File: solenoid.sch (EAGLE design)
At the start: 43 parts, among them U1 QS5K2TR, U2 QS5K2TR, U3 QS5K2TR, U4 QS5K2TR, U5 QS5K2TR, U6 QS5K2TR, Y1 ECS-80-S-4X

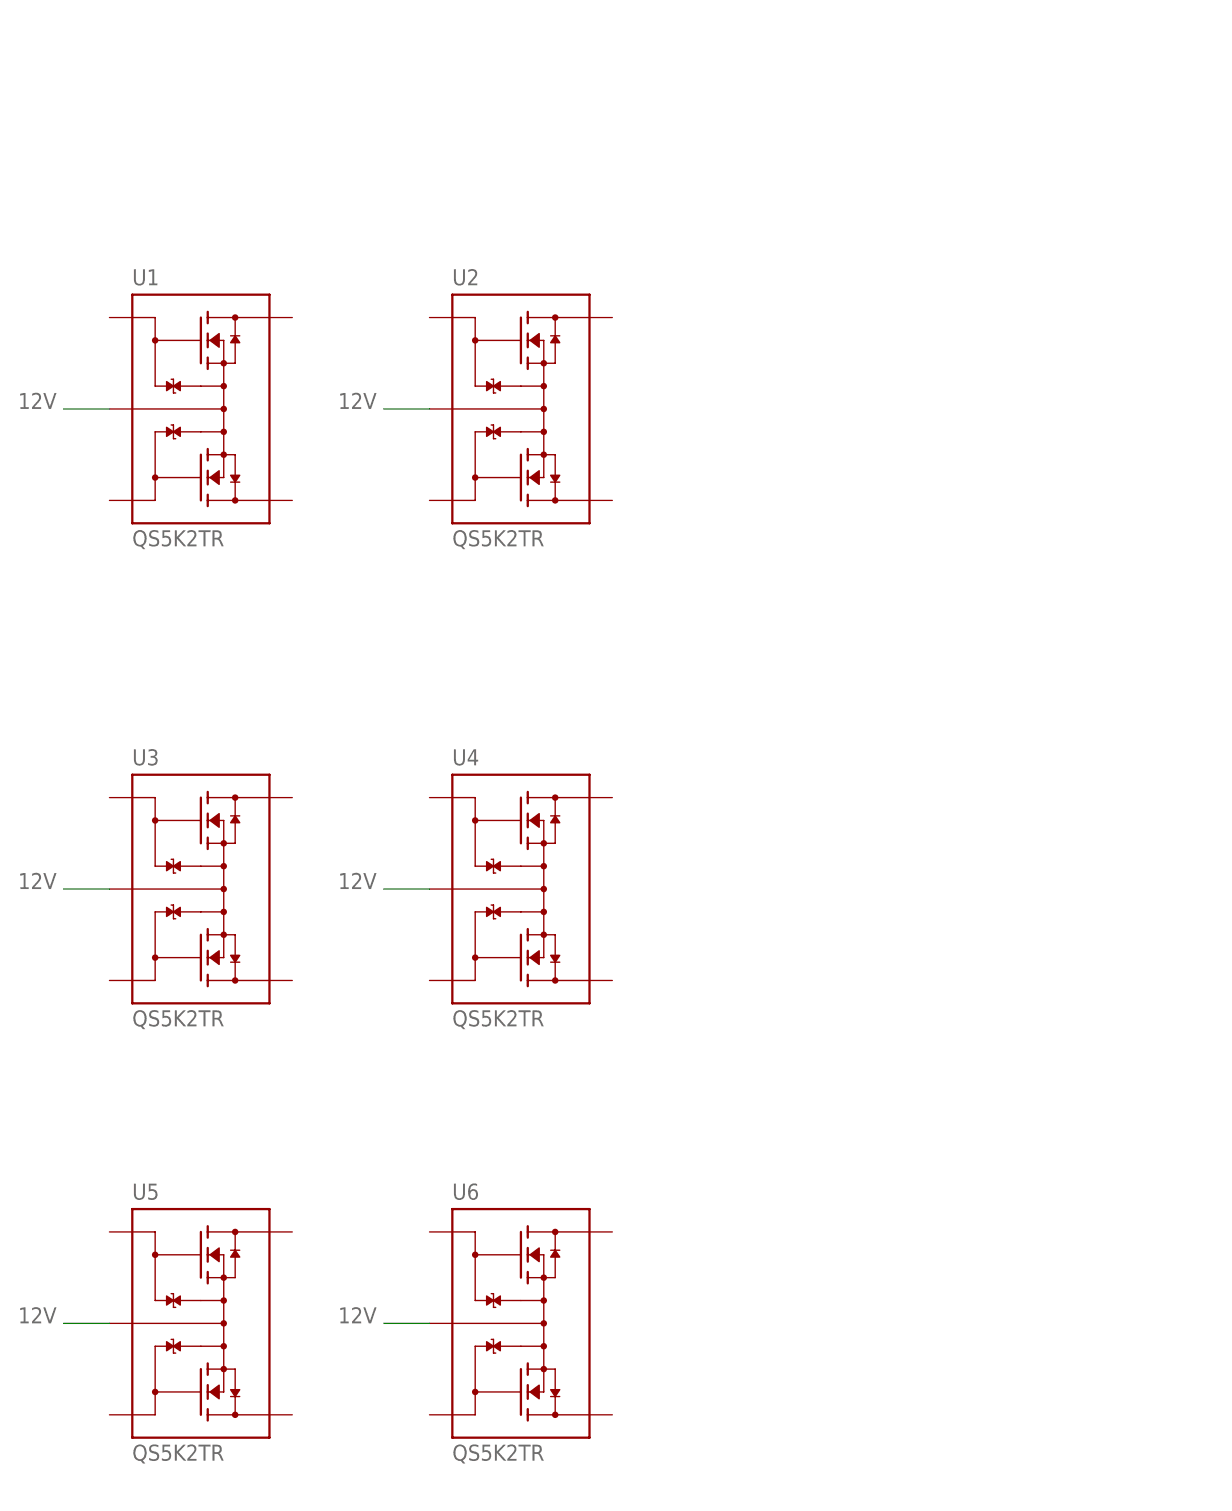
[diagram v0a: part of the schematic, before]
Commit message: potentially finished schematic
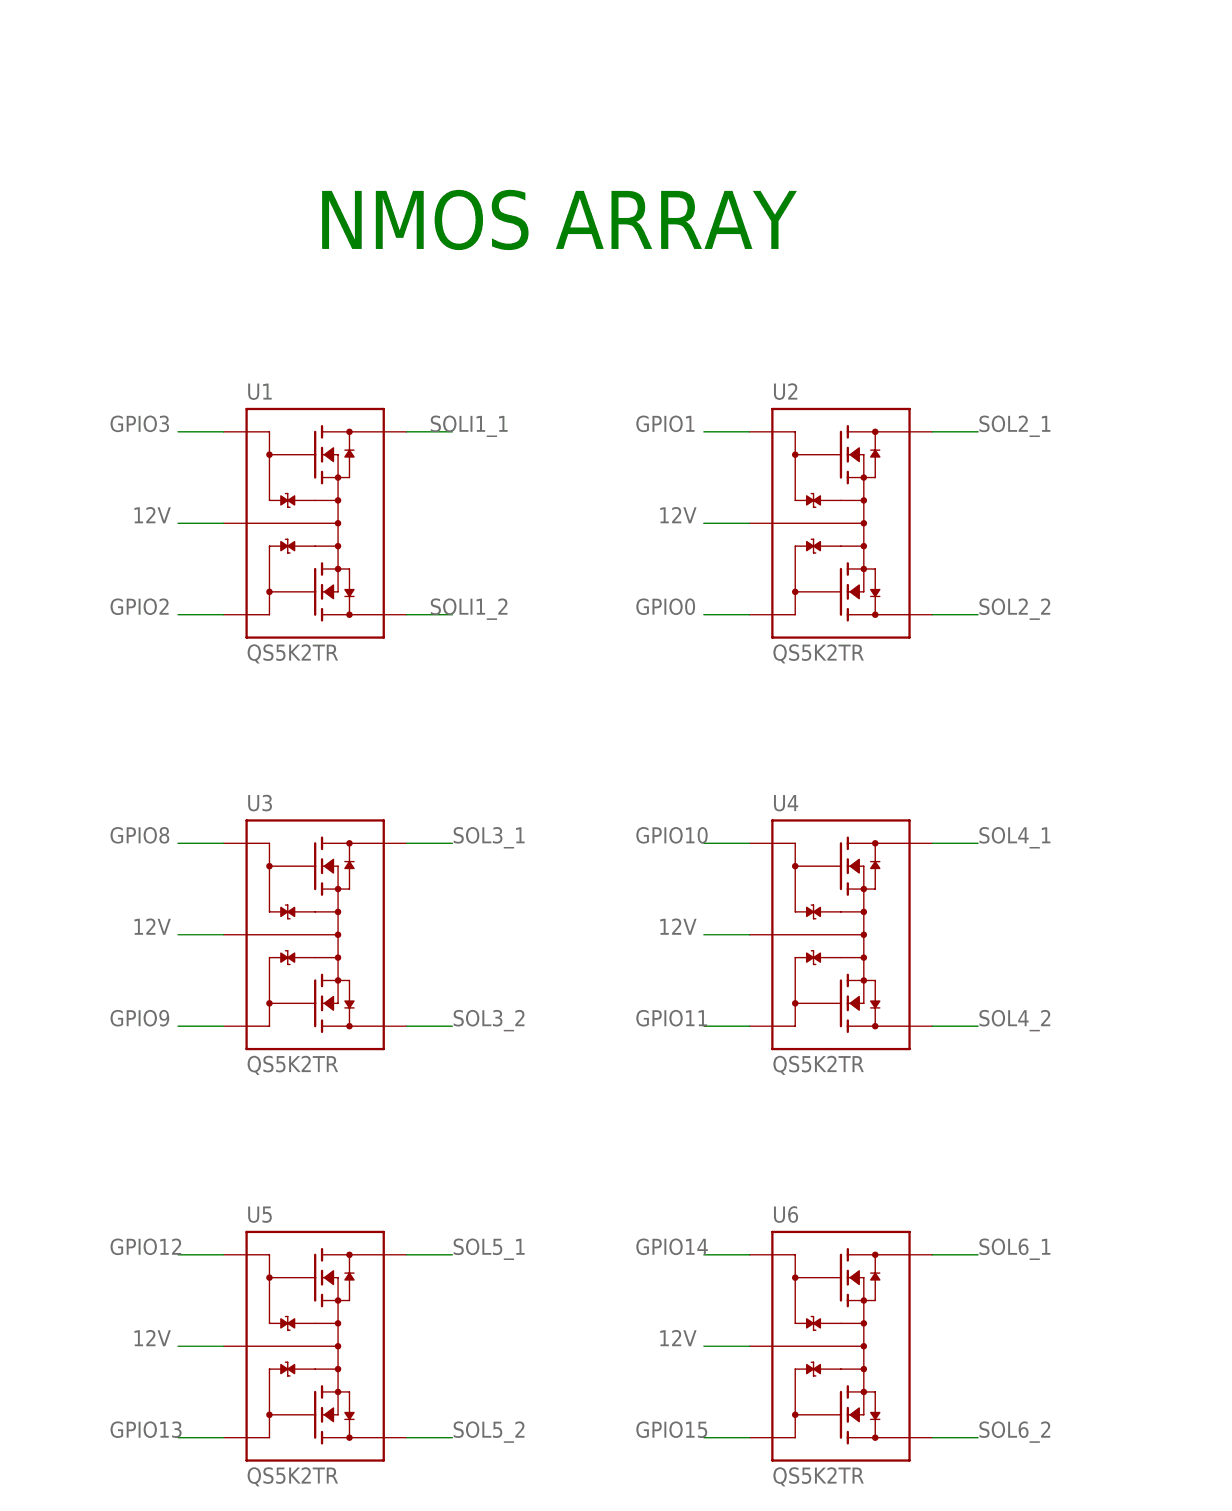
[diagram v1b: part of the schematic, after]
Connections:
- new net SOLI1_1: U1.TR1_DRAIN
- new net SOLI1_2: U1.TR2_DRAIN
- net GPIO0: now also U2.TR2_GATE
- net GPIO1: now also U2.TR1_GATE
- net GPIO10: now also U4.TR1_GATE
- net GPIO11: now also U4.TR2_GATE
- net GPIO12: now also U5.TR1_GATE
- net GPIO13: now also U5.TR2_GATE
- net GPIO14: now also U6.TR1_GATE
- net GPIO15: now also U6.TR2_GATE
- net GPIO2: now also U1.TR2_GATE
- net GPIO3: now also U1.TR1_GATE
- net GPIO8: now also U3.TR1_GATE
- net GPIO9: now also U3.TR2_GATE
- net SOL2_1: now also U2.TR1_DRAIN
- net SOL2_2: now also U2.TR2_DRAIN
- net SOL3_1: now also U3.TR1_DRAIN
- net SOL3_2: now also U3.TR2_DRAIN
- net SOL4_1: now also U4.TR1_DRAIN
- net SOL4_2: now also U4.TR2_DRAIN
- net SOL5_1: now also U5.TR1_DRAIN
- net SOL5_2: now also U5.TR2_DRAIN
- net SOL6_1: now also U6.TR1_DRAIN
- net SOL6_2: now also U6.TR2_DRAIN
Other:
- note added: "NMOS ARRAY"
- moved on the sheet: U1, U2, U3, U4, U5, U6

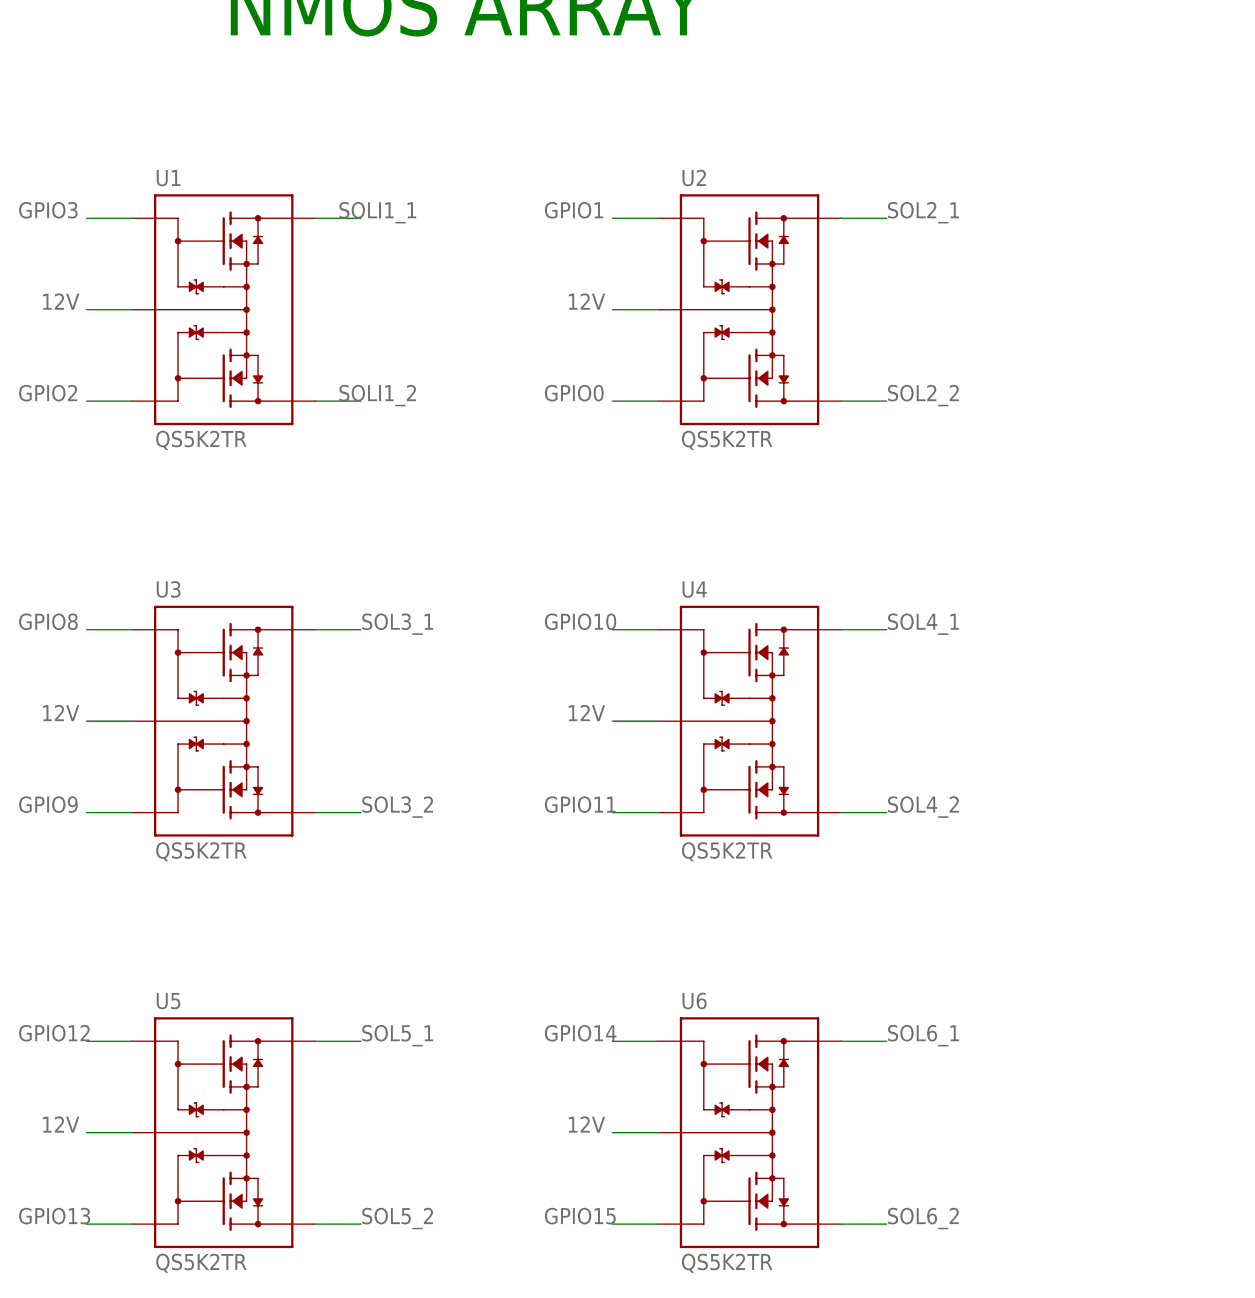
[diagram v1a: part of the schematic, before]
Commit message: solenoid work
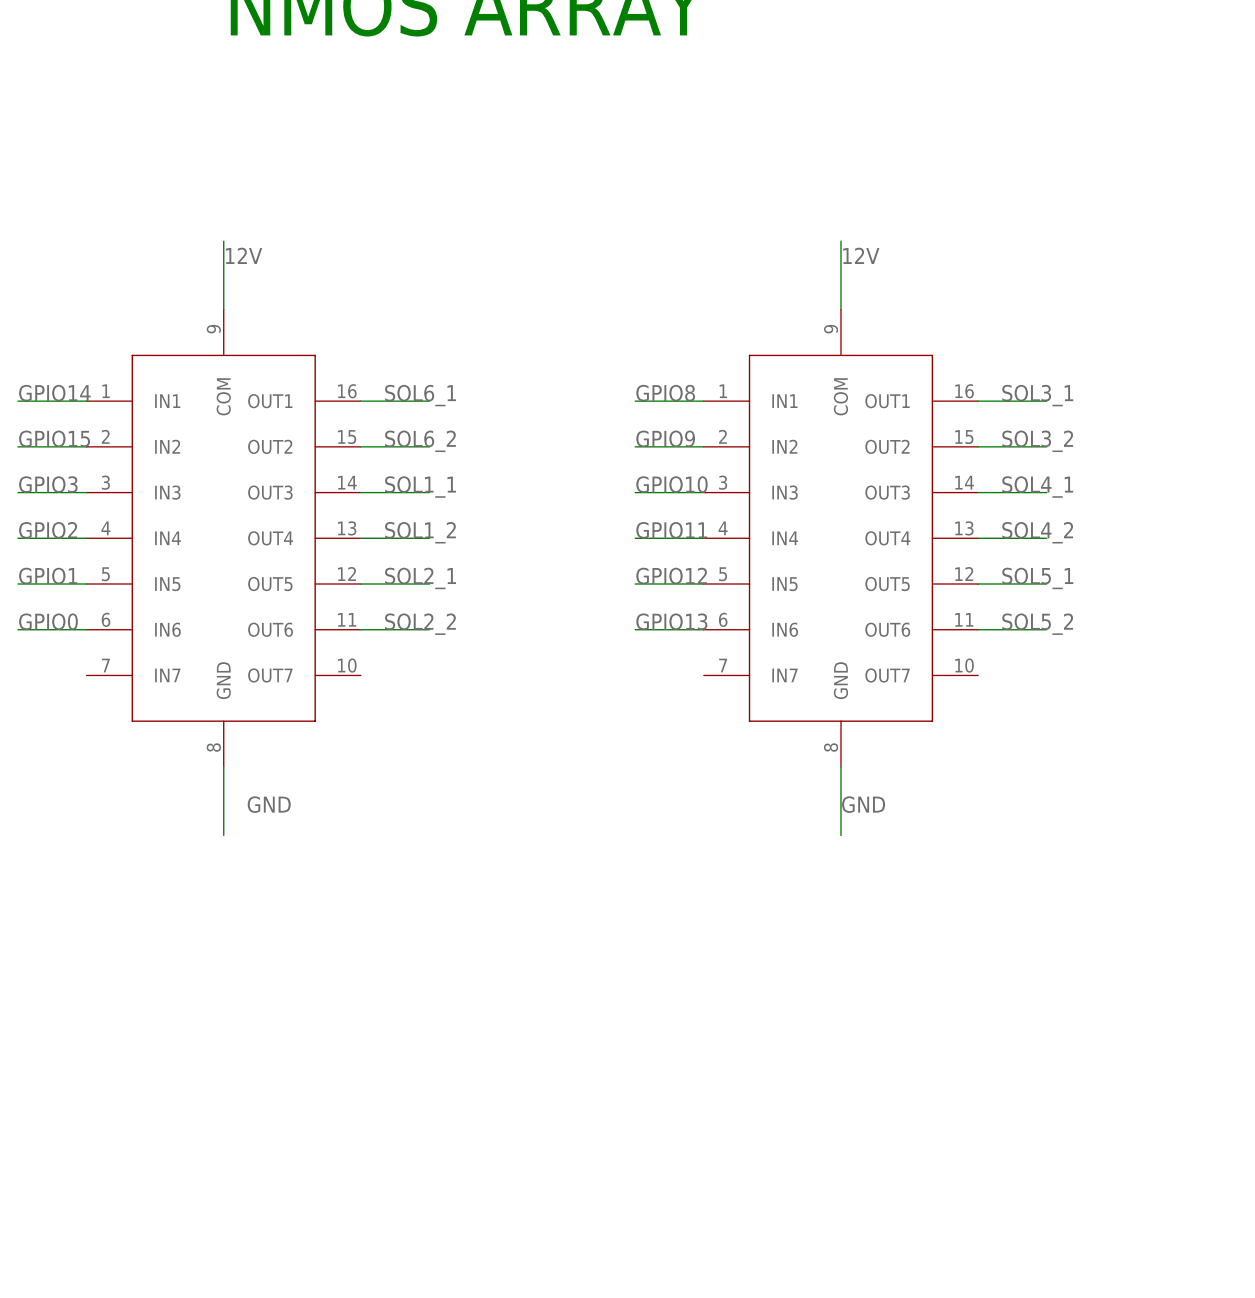
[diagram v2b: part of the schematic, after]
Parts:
- removed U3, U4, U5, U6: QS5K2TR, QS5K2TR:QS5K2TR
- U1, U2: value QS5K2TR -> ULN2003V12; device QS5K2TR:QS5K2TR -> ULN2003V12:ULN2003V12
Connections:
- removed net SOLI1_1: U1.TR1_DRAIN
- removed net SOLI1_2: U1.TR2_DRAIN
- net 12V: now also U1.COM, U2.COM; no longer U1.TR1_TR2_SOURCE, U2.TR1_TR2_SOURCE, U3.TR1_TR2_SOURCE, U4.TR1_TR2_SOURCE, U5.TR1_TR2_SOURCE, U6.TR1_TR2_SOURCE
- net GND: now also U1.GND, U2.GND
- net GPIO0: now also U1.IN6; no longer U2.TR2_GATE
- net GPIO1: now also U1.IN5; no longer U2.TR1_GATE
- net GPIO10: now also U2.IN3; no longer U4.TR1_GATE
- net GPIO11: now also U2.IN4; no longer U4.TR2_GATE
- net GPIO12: now also U2.IN5; no longer U5.TR1_GATE
- net GPIO13: now also U2.IN6; no longer U5.TR2_GATE
- net GPIO14: now also U1.IN1; no longer U6.TR1_GATE
- net GPIO15: now also U1.IN2; no longer U6.TR2_GATE
- net GPIO2: now also U1.IN4; no longer U1.TR2_GATE
- net GPIO3: now also U1.IN3; no longer U1.TR1_GATE
- net GPIO8: now also U2.IN1; no longer U3.TR1_GATE
- net GPIO9: now also U2.IN2; no longer U3.TR2_GATE
- net SOL1_1: now also U1.OUT3
- net SOL1_2: now also U1.OUT4
- net SOL2_1: now also U1.OUT5; no longer U2.TR1_DRAIN
- net SOL2_2: now also U1.OUT6; no longer U2.TR2_DRAIN
- net SOL3_1: now also U2.OUT1; no longer U3.TR1_DRAIN
- net SOL3_2: now also U2.OUT2; no longer U3.TR2_DRAIN
- net SOL4_1: now also U2.OUT3; no longer U4.TR1_DRAIN
- net SOL4_2: now also U2.OUT4; no longer U4.TR2_DRAIN
- net SOL5_1: now also U2.OUT5; no longer U5.TR1_DRAIN
- net SOL5_2: now also U2.OUT6; no longer U5.TR2_DRAIN
- net SOL6_1: now also U1.OUT1; no longer U6.TR1_DRAIN
- net SOL6_2: now also U1.OUT2; no longer U6.TR2_DRAIN

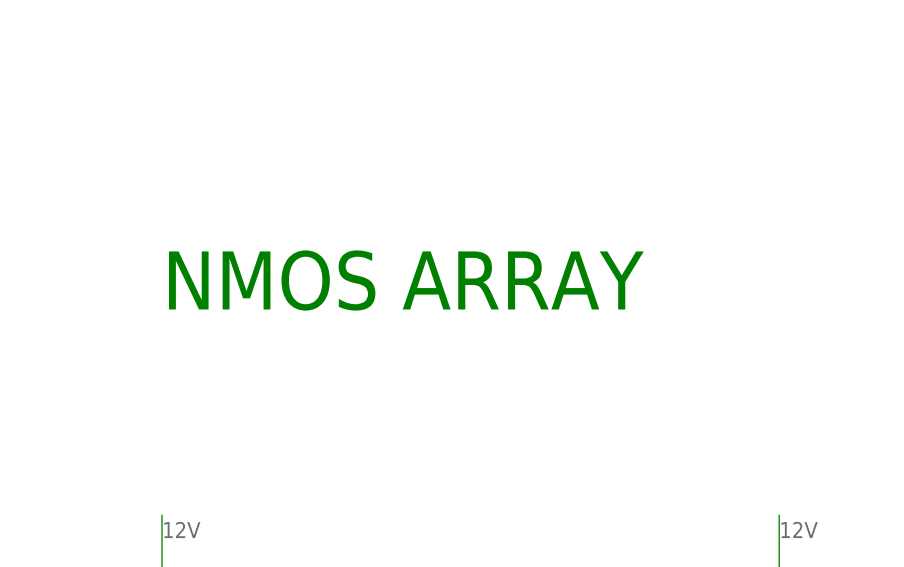
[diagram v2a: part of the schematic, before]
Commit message: uwu
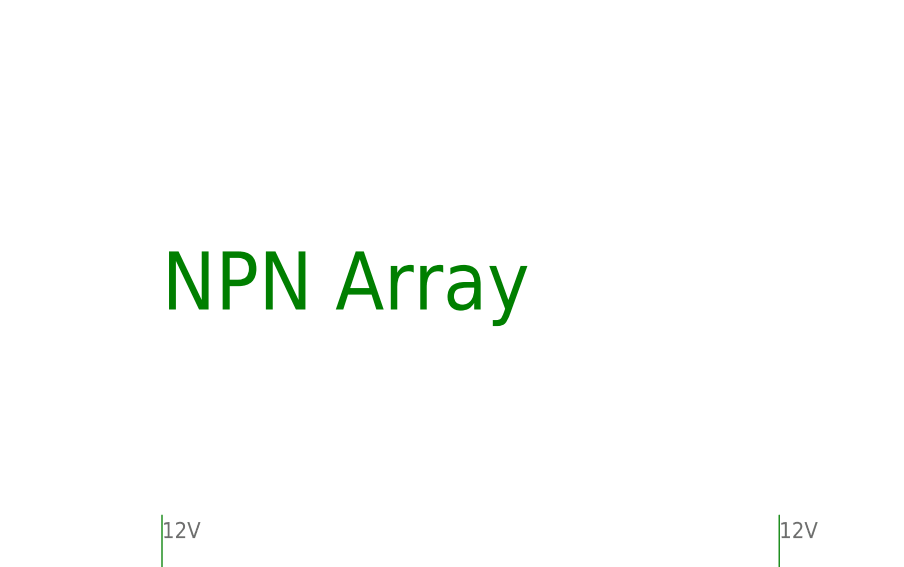
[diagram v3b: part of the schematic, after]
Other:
- note added: "NPN Array"
- note removed: "NMOS ARRAY"
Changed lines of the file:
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@@
 <text x="342.9" y="55.88" size="1.778" layer="91">Pin 5 (VDDA)</text>
 <text x="370.84" y="-33.02" size="5.08" layer="91">T21 Connector for 12V, CAN, GND</text>
-<text x="10.16" y="-17.78" size="6.4516" layer="91">NMOS ARRAY</text>
+<text x="10.16" y="-17.78" size="6.4516" layer="91">NPN Array</text>
 </plain>
 <instances>

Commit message: k
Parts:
- removed U2: ULN2003V12, ULN2003V12:ULN2003V12
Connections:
- removed net SOL1_2: J1.1, U1.OUT4
- removed net SOL2_2: J2.1, U1.OUT6
- removed net SOL3_2: J5.1, U2.OUT2
- removed net SOL4_2: J6.1, U2.OUT4
- removed net SOL5_2: J7.1, U2.OUT6
- removed net SOL6_2: J8.1, U1.OUT2
- new net GPIO4: U1.IN4
- new net GPIO5: U1.IN5
- new net GPIO6: U1.IN6
- net 12V: now also J1.1, J2.1, J5.1, J6.1, J7.1, J8.1; no longer U2.COM
- net GND: no longer U2.GND
- net GPIO0: no longer U1.IN6
- net GPIO1: now also U1.IN1; no longer U1.IN5
- net GPIO10: no longer U2.IN3
- net GPIO11: no longer U2.IN4
- net GPIO12: no longer U2.IN5
- net GPIO13: no longer U2.IN6
- net GPIO14: no longer U1.IN1
- net GPIO15: no longer U1.IN2
- net GPIO2: now also U1.IN2; no longer U1.IN4
- net GPIO8: no longer U2.IN1
- net GPIO9: no longer U2.IN2
- net SOL1_1: now also U1.OUT1; no longer U1.OUT3
- net SOL2_1: now also U1.OUT2; no longer U1.OUT5
- net SOL3_1: now also U1.OUT3; no longer U2.OUT1
- net SOL4_1: now also U1.OUT4; no longer U2.OUT3
- net SOL5_1: now also U1.OUT5; no longer U2.OUT5
- net SOL6_1: now also U1.OUT6; no longer U1.OUT1
